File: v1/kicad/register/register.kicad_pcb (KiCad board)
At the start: 2 copper layers, 127 x 104.5 mm, 5 parts, among them J3 ASYNC_{out}, U1 74HC173, U2 74HC173, U3 74LS244, U5 LNCPU Type B Connector

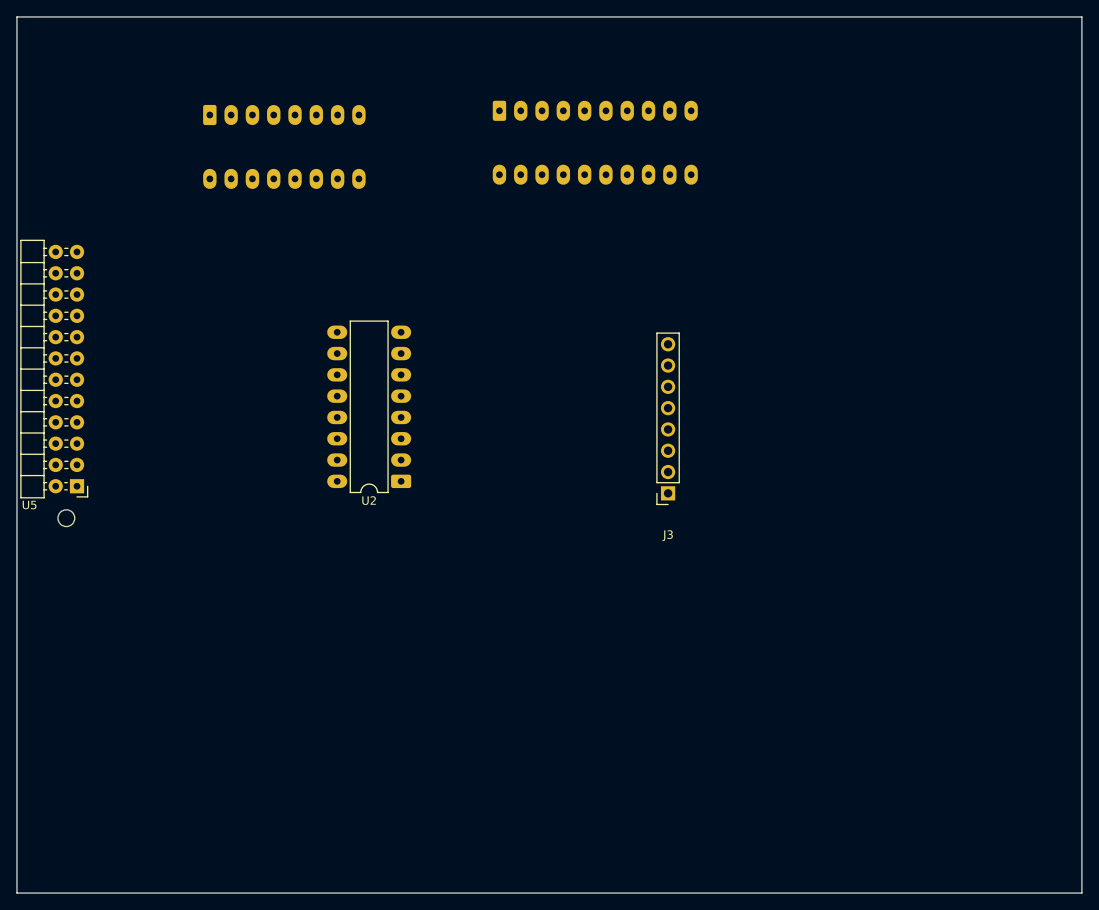
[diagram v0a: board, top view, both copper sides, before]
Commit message: partial
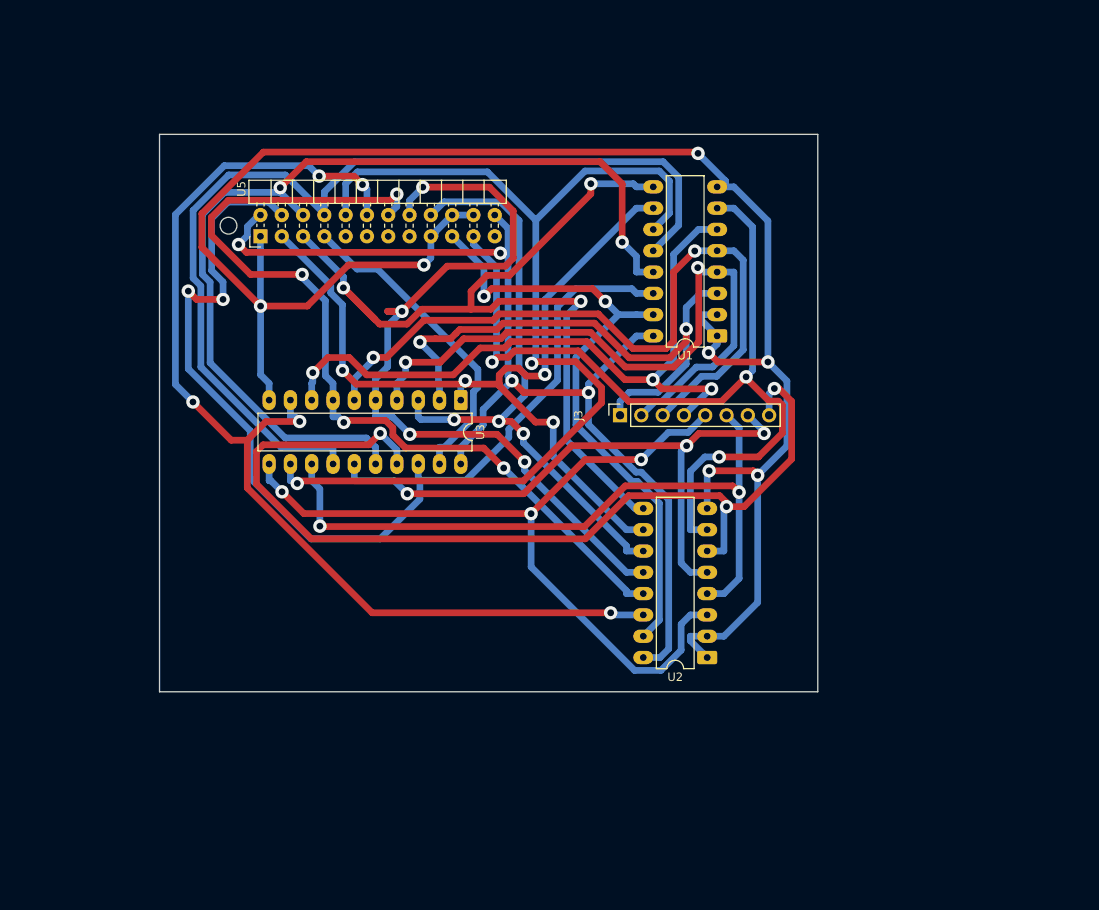
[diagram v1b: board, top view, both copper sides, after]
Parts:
- U1, U3: moved to F.Cu
- moved U1 66.0 mm to (101.5, 54.0), turned to 180 degrees
- moved U2 42.1 mm to (100.3, 92.4)
- moved U5 37.0 mm to (47.0, 42.2), turned to 90 degrees
- moved U3 34.8 mm to (70.9, 61.7)
- moved J3 10.9 mm to (89.9, 63.5), turned to 90 degrees
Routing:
- net Net-(U1-GND): track 0.00 -> 227.8 mm, vias 0 -> 7
- net /DBUS4: track 0.00 -> 130.8 mm, vias 0 -> 5
- net Net-(U1-VCC): track 0.00 -> 129.5 mm, vias 0 -> 4
- net /DBUS3: track 0.00 -> 126.8 mm, vias 0 -> 2
- net /DBUS0: track 0.00 -> 122.7 mm, vias 0 -> 2
- net Net-(U1-E1): track 0.00 -> 120.3 mm, vias 0 -> 3
- net /DBUS2: track 0.00 -> 117.5 mm
- net /ASYNC7: track 0.00 -> 116.3 mm, vias 0 -> 3
- net /DBUS1: track 0.00 -> 115.1 mm, vias 0 -> 2
- net /DBUS5: track 0.00 -> 106.2 mm, vias 0 -> 4
- net Net-(U1-Cp): track 0.00 -> 105.2 mm, vias 0 -> 3
- net Net-(U1-E2): track 0.00 -> 101.9 mm, vias 0 -> 4
- net /DBUS6: track 0.00 -> 98.4 mm, vias 0 -> 4
- net /ASYNC4: track 0.00 -> 97.5 mm, vias 0 -> 3
- net /ASYNC2: track 0.00 -> 87.8 mm, vias 0 -> 2
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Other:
- board size 127 x 104.5 mm -> 78.5 x 66.5 mm
